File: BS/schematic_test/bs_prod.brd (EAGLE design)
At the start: 84 x 49 mm, 21 parts, among them U1 ATMEGA328P_PDIP, U2 RFM69HW, Y1 16MHz

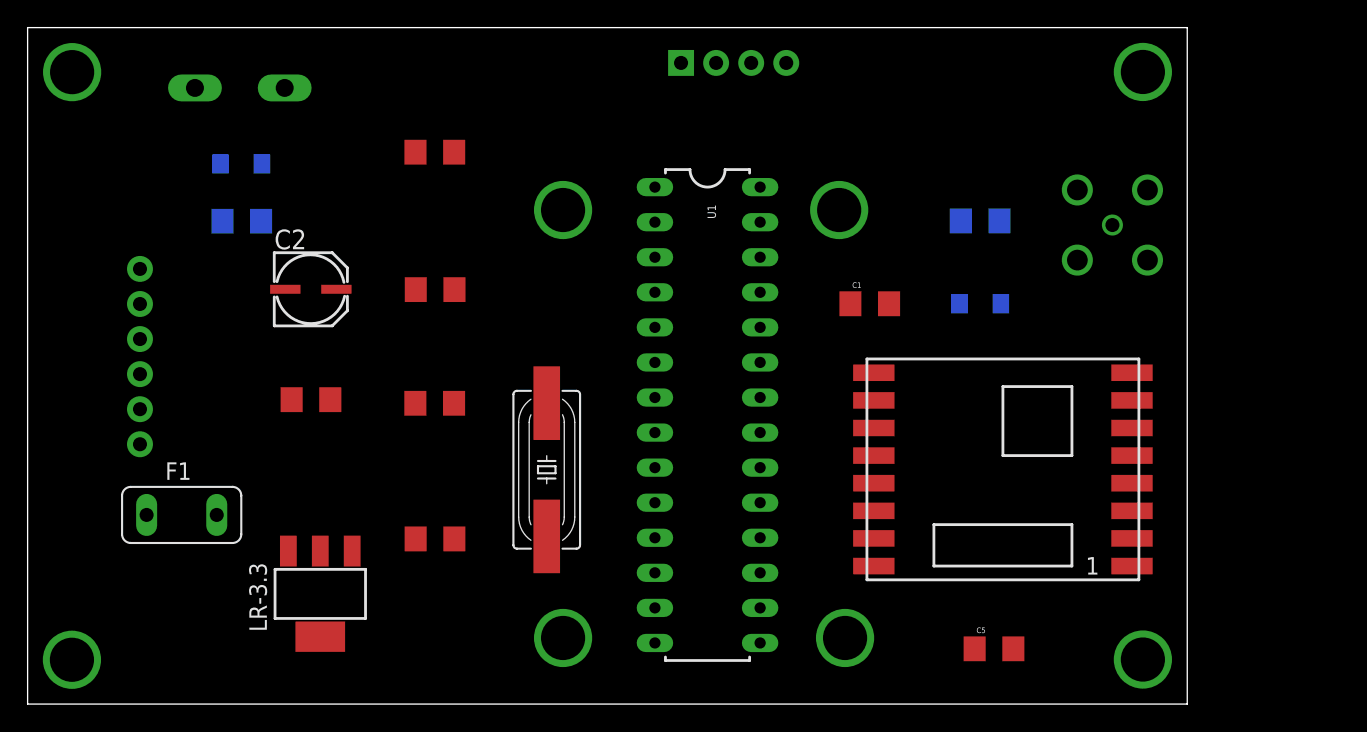
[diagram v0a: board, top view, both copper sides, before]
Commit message: BS schematic prod
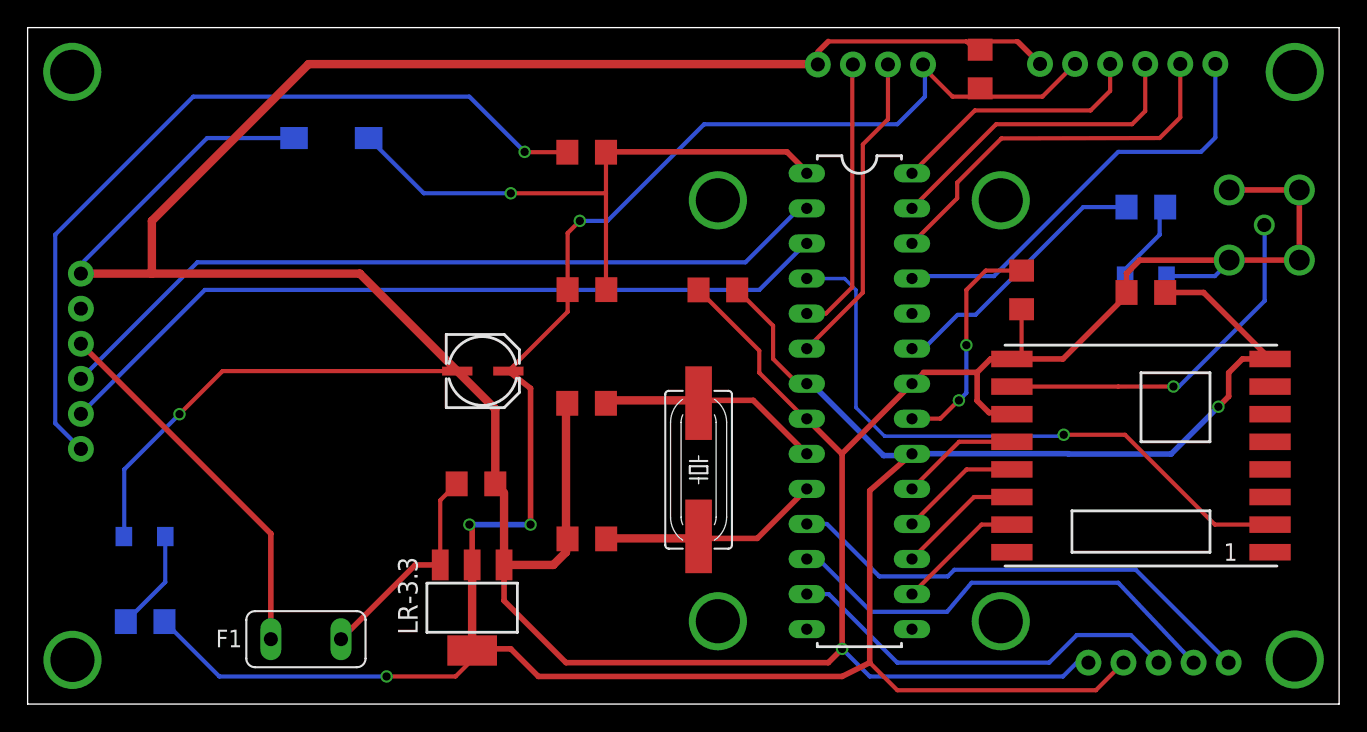
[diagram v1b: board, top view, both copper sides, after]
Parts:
- removed LED1: (no value), SparkFun-LED:LED-1206
- removed S1: DTS-3, switch-tact:DTS-3
- added C8, C9: 0.1uF, SparkFun-Capacitors:1206
- added JP3: (no value), SparkFun-Connectors:1X06
- added JP4: (no value), SparkFun-Connectors:1X05
- added PWR: (no value), SparkFun-LED:LED-1206
- added RESET: DTSM-3, switch-tact:DTSM-3
- added U$1: UBLOX, myGps:UBLOX
- C2: value (none) -> 10uF
- moved R2 29.8 mm to (8.51, 5.97)
- moved C5 28.1 mm to (81.0, 29.8), turned to 180 degrees
- moved C2 13.8 mm to (32.9, 24.3)
- moved JP1 13.7 mm to (3.86, 18.5), turned to 90 degrees
- moved C7 13.4 mm to (32.5, 16.0), turned to 0 degrees
- moved F1 12.7 mm to (20.2, 4.70)
- moved LED2 12.2 mm to (81.0, 31.0)
- moved R3 12.0 mm to (81.0, 36.0)
- moved LR-3.3 11.0 mm to (32.2, 6.98)
- moved C1 11.0 mm to (72.0, 30.0), turned to 270 degrees
- moved U1 11.0 mm to (60.3, 21.9)
- moved C3 11.0 mm to (40.5, 21.8)
- moved C6 11.0 mm to (40.5, 40.0)
- moved C4 11.0 mm to (40.5, 12.0)
- moved SMA 11.0 mm to (89.6, 34.7)
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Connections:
- new net A0: JP3.4, U1.28
- new net A1: JP3.3, U1.27
- new net A2: JP3.2, U1.26
- new net A3: JP3.1, U1.25
- new net D5: JP4.1, U1.11
- new net D6: JP4.2, U1.12
- new net D7: JP4.3, U1.13
- net 3.3V: now also C8.1, C9.1, JP3.5, JP4.4
- net GND: now also C8.2, C9.2, JP3.6, JP4.5, PWR.C, RESET.2; no longer LED1.C, S1.2
- net N$5: now also PWR.A; no longer LED1.A
- net RST: now also RESET.1; no longer S1.1
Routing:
- net GND: track 0.00 -> 335.6 mm, vias 0 -> 2
- net 3.3V: track 0.00 -> 233.8 mm, vias 0 -> 5
- net N$11: track 0.00 -> 59.2 mm, vias 0 -> 1
- net D0_RX: track 0.00 -> 57.7 mm
- net D1_TX: track 0.00 -> 57.7 mm
- net D2: track 0.00 -> 46.0 mm, vias 0 -> 1
- net RST: track 0.00 -> 44.1 mm, vias 0 -> 1
- net D5: track 0.00 -> 35.1 mm
- net D6: track 0.00 -> 33.1 mm
- net A3: track 0.00 -> 31.5 mm
- net D7: track 0.00 -> 29.2 mm
- net A2: track 0.00 -> 27.7 mm
- net N$9: track 0.00 -> 27.1 mm
- net N$8: track 0.00 -> 26.4 mm, vias 0 -> 1
- net A1: track 0.00 -> 23.2 mm
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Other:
- board size 84 x 49 mm -> 95 x 49 mm
- board text added: "+5V"
- board text added: "3V3"
- board text added: "A2"
- board text added: "A3"
- board text added: "CTS"
- board text added: "D5"
- board text added: "D6"
- board text added: "D7"
- board text added: "DTR"
- board text added: "GND"
- board text added: "Matsepura A.M. MAI 07-608"
- board text added: "RX"
- board text added: "SCL"
- board text added: "SDA"
- board text added: "TX"
- board text added: "TX\"
